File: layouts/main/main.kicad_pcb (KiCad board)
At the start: 4 copper layers, 20.5 x 20.5 mm, 60 parts

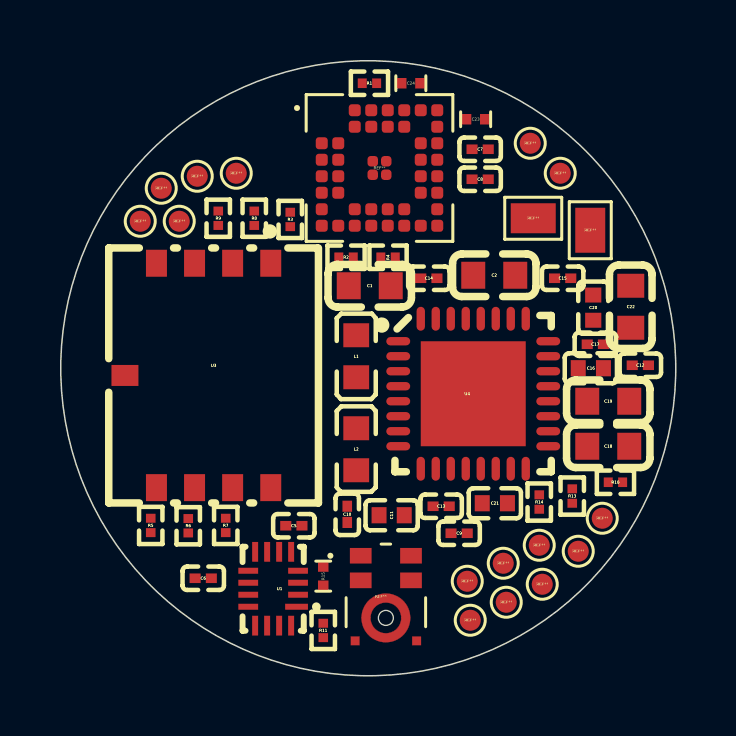
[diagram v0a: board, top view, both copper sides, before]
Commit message: wip
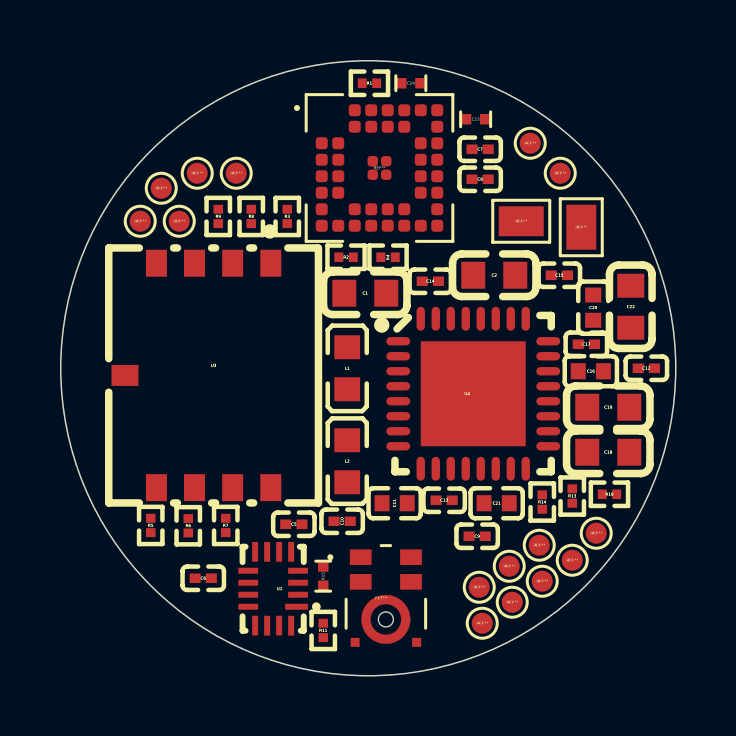
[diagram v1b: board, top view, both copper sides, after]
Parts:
- moved C9 0.61 mm to (3.63, 5.60)
- moved REF** 0.54 mm to (7.60, 5.50)
- moved L1 0.50 mm to (-0.70, 0.00)
- moved L2 0.50 mm to (-0.70, 3.10)
- moved R10 0.45 mm to (8.04, 4.20)
- moved REF** 0.45 mm to (3.70, 7.30)
- moved C11 0.41 mm to (0.88, 4.50)
- moved REF** 0.41 mm to (5.10, -4.90)
- moved REF** 0.41 mm to (3.80, 8.50)
- moved REF** 0.36 mm to (6.80, 6.40)
- moved REF** 0.32 mm to (7.10, -4.70)
- moved C17 0.30 mm to (7.27, -0.80)
- moved C1 0.29 mm to (-0.10, -2.50)
- moved C10 0.29 mm to (-0.87, 5.10), turned to 180 degrees
- moved REF** 0.22 mm to (4.70, 6.60)
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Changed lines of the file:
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@@
 	(footprint "POGO_PAD:POGO_PAD"
 		(layer "F.Cu")
-		(at 7.8 5)
+		(at 7.6 5.5)
 		(property "Reference" "REF**"
 			(at 0 0 0)
@@
 	(footprint "UNI_ROYAL_0201WMF0000TEE:R0201"
 		(layer "F.Cu")
-		(at 8.24 3.8)
+		(at 8.04 4.2)
 		(property "Reference" "R10"
 			(at 0 0 0)
@@
 	(footprint "UNI_ROYAL_0201WMF1002TEE:R0201"
 		(layer "F.Cu")
-		(at -3.8 -5 90)
+		(at -3.9 -5.06 90)
 		(property "Reference" "R8"
 			(at 0 0 0)
@@
 	(footprint "POGO_PAD:POGO_PAD"
 		(layer "F.Cu")
-		(at 3.3 7.1)
+		(at 3.7 7.3)
 		(property "Reference" "REF**"
 			(at 0 0 0)
@@
 	(footprint "Samsung_Electro_Mechanics_CL10A106KP8NNNC:C0603"
 		(layer "F.Cu")
-		(at 8 2.6)
+		(at 8 2.8)
 		(property "Reference" "C18"
 			(at 0 0 0)
@@
 	(footprint "Murata_Electronics_GRM033R60J104KE19D:C0201"
 		(layer "F.Cu")
-		(at -0.7 4.87 -90)
+		(at -0.87 5.1 180)
 		(property "Reference" "C10"
-			(at 0 -0.000167 0)
+			(at 0 -0.000167 90)
 			(layer "F.SilkS")
 			(effects
@@
 		)
 		(property "Value" "100nF ±10% X5R"
-			(at 0 -0.000167 0)
+			(at 0 -0.000167 90)
 			(layer "F.Fab")
 			(effects
@@
 		)
 		(property "Datasheet" "https://wmsc.lcsc.com/wmsc/upload/file/pdf/v2/lcsc/2304140030_Murata-Electronics-GRM033R60J104KE19D_C76928.pdf"
-			(at 0 0 90)
+			(at 0 0 0)
 			(layer "User.9")
 			(hide yes)
@@
 		)
 		(property "Description" ""
-			(at 0 0 90)
+			(at 0 0 0)
 			(layer "F.Fab")
 			(hide yes)
@@
 		)
 		(property "checksum" "4c698f746e469e1dee8eb9906937a259cc1e41bf0b356ab1e01eb74657f75796"
-			(at 0 0 0)
+			(at 0 0 90)
 			(layer "User.9")
 			(hide yes)
@@
 		)
 		(property "__atopile_lib_fp_hash__" "0fb5227f-9857-c04c-e64f-3cbb1c0819d1"
-			(at 0 0 0)
+			(at 0 0 90)
 			(layer "User.9")
 			(hide yes)
@@
 		)
 		(property "LCSC" "C76928"
-			(at 0 0 90)
+			(at 0 0 0)
 			(layer "User.9")
 			(hide yes)
@@
 		)
 		(property "Manufacturer" "Murata Electronics"
-			(at 0 0 90)
+			(at 0 0 0)
 			(layer "User.9")
 			(hide yes)
@@
 		)
 		(property "Partnumber" "GRM033R60J104KE19D"
-			(at 0 0 90)
+			(at 0 0 0)
 			(layer "User.9")
 			(hide yes)
@@
 		)
 		(property "PARAM_capacitance" "{\"type\": \"Quantity_Interval_Disjoint\", \"data\": {\"intervals\": {\"type\": \"Numeric_Interval_Disjoint\", \"data\": {\"intervals\": [{\"type\": \"Numeric_Interval\", \"data\": {\"min\": 9e-08, \"max\": 1.1e-07}}]}}, \"unit\": \"farad\"}}"
-			(at 0 0 90)
+			(at 0 0 0)
 			(layer "User.9")
 			(hide yes)
@@
 		)
 		(property "PARAM_max_voltage" "{\"type\": \"Quantity_Interval_Disjoint\", \"data\": {\"intervals\": {\"type\": \"Numeric_Interval_Disjoint\", \"data\": {\"intervals\": [{\"type\": \"Numeric_Interval\", \"data\": {\"min\": 0.0, \"max\": null}}]}}, \"unit\": \"volt\"}}"
-			(at 0 0 90)
+			(at 0 0 0)
 			(layer "User.9")
 			(hide yes)
@@
 		)
 		(property "PARAM_temperature_coefficient" "{\"type\": \"EnumSet\", \"data\": {\"elements\": [{\"name\": \"X5R\"}], \"enum\": {\"name\": \"TemperatureCoefficient\", \"values\": {\"Y5V\": 1, \"Z5U\": 2, \"X7S\": 3, \"X5R\": 4, \"X6R\": 5, \"X7R\": 6, \"X8R\": 7, \"C0G\": 8}}}}"
-			(at 0 0 90)
+			(at 0 0 0)
 			(layer "User.9")
 			(hide yes)
@@
 		)
 		(property "atopile_address" "c_nand"
-			(at 0 0 90)
+			(at 0 0 0)
 			(layer "User.9")
 			(hide yes)
@@
 		(attr through_hole)
 		(fp_line
-			(start -0.17 0.39)
-			(end -0.53 0.39)
+			(start 0.69 0.24)
+			(end 0.69 -0.24)
 			(stroke
 				(width 0.15)
@@
 		)
 		(fp_line
-			(start 0.17 0.39)
-			(end 0.53 0.39)
+			(start 0.53 -0.39)
+			(end 0.17 -0.39)
 			(stroke
 				(width 0.15)
@@
 		)
 		(fp_line
-			(start -0.69 0.24)
-			(end -0.69 -0.24)
+			(start 0.17 0.39)
+			(end 0.53 0.39)
 			(stroke
 				(width 0.15)
@@
 		)
 		(fp_line
-			(start 0.69 0.24)
-			(end 0.69 -0.24)
+			(start -0.17 0.39)
+			(end -0.53 0.39)
 			(stroke
 				(width 0.15)
@@
 		)
 		(fp_line
-			(start 0.53 -0.39)
-			(end 0.17 -0.39)
+			(start -0.69 0.24)
+			(end -0.69 -0.24)
 			(stroke
 				(width 0.15)
@@
 		)
 		(fp_arc
-			(start -0.529667 0.389644)
-			(mid -0.642347 0.349658)
-			(end -0.69 0.24)
+			(start 0.69 0.24)
+			(mid 0.642348 0.349658)
+			(end 0.529667 0.389644)
 			(stroke
 				(width 0.15)
@@
 		)
 		(fp_arc
-			(start 0.69 0.24)
-			(mid 0.642348 0.349658)
-			(end 0.529667 0.389644)
+			(start 0.53 -0.39)
+			(mid 0.642835 -0.349658)
+			(end 0.690333 -0.239643)
 			(stroke
 				(width 0.15)
@@
 		)
 		(fp_arc
-			(start -0.690333 -0.239643)
-			(mid -0.642835 -0.349658)
-			(end -0.53 -0.39)
+			(start -0.529667 0.389644)
+			(mid -0.642347 0.349658)
+			(end -0.69 0.24)
 			(stroke
 				(width 0.15)
@@
 		)
 		(fp_arc
-			(start 0.53 -0.39)
-			(mid 0.642835 -0.349658)
-			(end 0.690333 -0.239643)
+			(start -0.690333 -0.239643)
+			(mid -0.642835 -0.349658)
+			(end -0.53 -0.39)
 			(stroke
 				(width 0.15)
@@
 		)
 		(fp_text user "${REFERENCE}"
-			(at 0 -0.000167 0)
+			(at 0 -0.000167 90)
 			(layer "F.SilkS")
 			(effects
@@
 		)
 		(fp_text user "${REFERENCE}"
-			(at 0 -0.000167 0)
+			(at 0 -0.000167 90)
 			(layer "F.Fab")
 			(effects
@@
 		)
 		(pad "1" smd rect
-			(at -0.27 0 270)
+			(at -0.27 0 180)
 			(size 0.37 0.32)
 			(layers "F.Cu" "F.Mask" "F.Paste")
@@
 		)
 		(pad "2" smd rect
-			(at 0.27 0 270)
+			(at 0.27 0 180)
 			(size 0.37 0.32)
 			(layers "F.Cu" "F.Mask" "F.Paste")
@@
 	(footprint "Murata_Electronics_GRM033R60J104KE19D:C0201"
 		(layer "F.Cu")
-		(at 3.03 5.5)
+		(at 3.63 5.6)
 		(property "Reference" "C9"
 			(at 0 -0.000167 0)
@@
 	(footprint "POGO_PAD:POGO_PAD"
 		(layer "F.Cu")
-		(at 7 6.1)
+		(at 6.8 6.4)
 		(property "Reference" "REF**"
 			(at 0 0 0)
@@
 	(footprint "YAGEO_RC0201FR_07150KL:R0201"
 		(layer "F.Cu")
-		(at 5.7 4.46 -90)
+		(at 5.8 4.46 -90)
 		(property "Reference" "R14"
 			(at 0 0 0)
@@
 	(footprint "Murata_Electronics_GRM033R60J104KE19D:C0201"
 		(layer "F.Cu")
-		(at 2.02 -3)
+		(at 2.07 -2.9)
 		(property "Reference" "C14"
 			(at 0 -0.000167 0)
@@
 	(footprint "FH_CMH160808B2R2MT:L0603"
 		(layer "F.Cu")
-		(at -0.4 -0.4 90)
+		(at -0.7 0 90)
 		(property "Reference" "L1"
 			(at -0.005 0 0)
@@
 	(footprint "Murata_Electronics_GRM033R60J104KE19D:C0201"
 		(layer "F.Cu")
-		(at 2.43 4.6 180)
+		(at 2.53 4.4 180)
 		(property "Reference" "C13"
 			(at 0 -0.000166 0)
@@
 	(footprint "POGO_PAD:POGO_PAD"
 		(layer "F.Cu")
-		(at 4.6 7.8)
+		(at 4.8 7.8)
 		(property "Reference" "REF**"
 			(at 0 0 0)
@@
 	(footprint "UNI_ROYAL_0201WMF4701TEE:R0201"
 		(layer "F.Cu")
-		(at -2.6 -4.96 -90)
+		(at -2.7 -5.06 -90)
 		(property "Reference" "R3"
 			(at 0 0 0)
@@
 	(footprint "POGO_PAD:POGO_PAD"
 		(layer "F.Cu")
-		(at -5.7 -6.4)
+		(at -5.7 -6.5)
 		(property "Reference" "REF**"
 			(at 0 0 0)
@@
 	(footprint "Samsung_Electro_Mechanics_CL05A225MQ5NSNC:C0402"
 		(layer "F.Cu")
-		(at 0.78 4.9)
+		(at 0.88 4.5)
 		(property "Reference" "C11"
 			(at 0 0 90)
@@
 	(footprint "POGO_PAD:POGO_PAD"
 		(layer "F.Cu")
-		(at 4.5 6.5)
+		(at 4.7 6.6)
 		(property "Reference" "REF**"
 			(at 0 0 0)
@@
 	(footprint "Samsung_Electro_Mechanics_CL05A105KA5NQNC:C0402"
 		(layer "F.Cu")
-		(at 4.22 4.5)
+		(at 4.28 4.5)
 		(property "Reference" "C21"
 			(at 0 0 0)
@@
 	(footprint "FH_CMH160808B2R2MT:L0603"
 		(layer "F.Cu")
-		(at -0.4 2.7 -90)
+		(at -0.7 3.1 -90)
 		(property "Reference" "L2"
 			(at -0.005 0 0)
@@
 	(footprint "INVENSENSE_MMICT5838_00_012:MIC_T5838"
 		(layer "F.Cu")
-		(at 0.5875 7.612)
+		(at 0.5875 7.662)
 		(property "Reference" "REF**"
 			(at -0.1625 0 0)
@@
 	(footprint "Samsung_Electro_Mechanics_CL05A105KA5NQNC:C0402"
 		(layer "F.Cu")
-		(at 7.42 0)
+		(at 7.42 0.1)
 		(property "Reference" "C16"
 			(at 0 0 0)
@@
 	(footprint "Murata_Electronics_GRM033R60J104KE19D:C0201"
 		(layer "F.Cu")
-		(at 9.07 -0.1)
+		(at 9.27 0)
 		(property "Reference" "C12"
 			(at 0 -0.000167 0)
@@
 	(footprint "Samsung_Electro_Mechanics_CL10A106KP8NNNC:C0603"
 		(layer "F.Cu")
-		(at 8 1.1)
+		(at 8 1.3)
 		(property "Reference" "C19"
 			(at 0 0 0)
@@
 	(footprint "BATTERY_PAD:BATTERY_PAD"
 		(layer "F.Cu")
-		(at 7.4 -4.6 180)
+		(at 7.1 -4.7 180)
 		(property "Reference" "REF**"
 			(at 0 0 0)
@@
 	(footprint "POGO_PAD:POGO_PAD"
 		(layer "F.Cu")
-		(at 3.4 8.4)
+		(at 3.8 8.5)
 		(property "Reference" "REF**"
 			(at 0 0 0)
@@
 	(footprint "Murata_Electronics_GRM033R60J104KE19D:C0201"
 		(layer "F.Cu")
-		(at 6.48 -3)
+		(at 6.37 -3.1)
 		(property "Reference" "C15"
 			(at 0 -0.000167 0)
@@
 	(footprint "POGO_PAD:POGO_PAD"
 		(layer "F.Cu")
-		(at 5.8 7.2)
+		(at 5.8 7.1)
 		(property "Reference" "REF**"
 			(at 0 0 0)
@@
 	(footprint "Samsung_Electro_Mechanics_CL10A106KP8NNNC:C0603"
 		(layer "F.Cu")
-		(at 0.05 -2.75)
+		(at -0.1 -2.5)
 		(property "Reference" "C1"
 			(at 0 0 0)
@@
 	(footprint "Murata_Electronics_GRM033R60J104KE19D:C0201"
 		(layer "F.Cu")
-		(at 7.57 -0.8)
+		(at 7.27 -0.8)
 		(property "Reference" "C17"
 			(at 0 -0.000167 0)
@@
 	(footprint "Murata_Electronics_GRM033R60J104KE19D:C0201"
 		(layer "F.Cu")
-		(at -2.48 5.25)
+		(at -2.48 5.2)
 		(property "Reference" "C5"
 			(at 0 -0.000167 0)
@@
 	(footprint "UNI_ROYAL_0201WMF1002TEE:R0201"
 		(layer "F.Cu")
-		(at -5 -5 90)
+		(at -5 -5.06 90)
 		(property "Reference" "R9"
 			(at 0 0 0)
@@
 	(footprint "BATTERY_PAD:BATTERY_PAD"
 		(layer "F.Cu")
-		(at 5.5 -5 -90)
+		(at 5.1 -4.9 -90)
 		(property "Reference" "REF**"
 			(at 0 0 0)

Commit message: drc rules
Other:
- rule pad_to_mask_clearance: 0 -> 0.05
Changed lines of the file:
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@@
 			(dielectric_constraints no)
 		)
-		(pad_to_mask_clearance 0)
+		(pad_to_mask_clearance 0.05)
+		(solder_mask_min_width 0.1)
 		(allow_soldermask_bridges_in_footprints no)
 		(tenting front back)

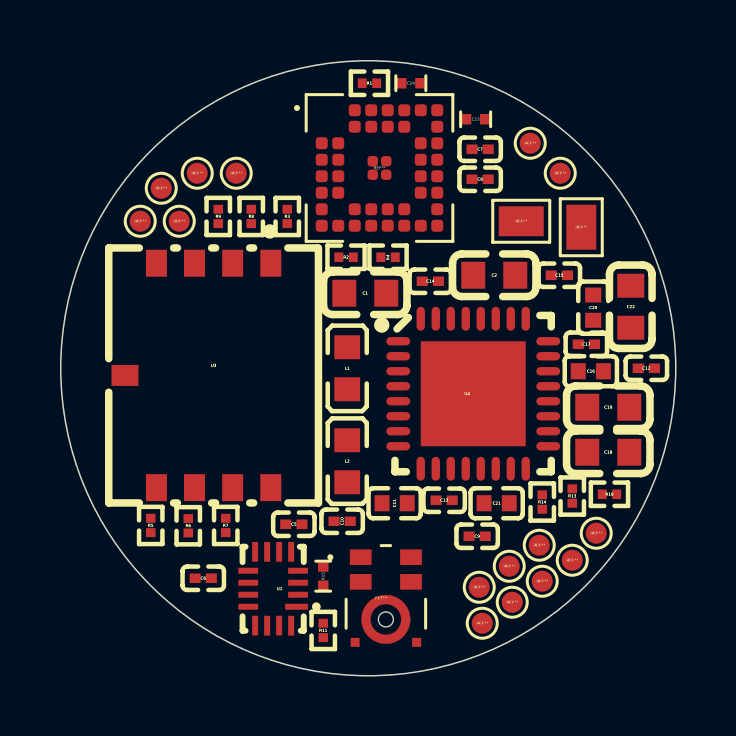
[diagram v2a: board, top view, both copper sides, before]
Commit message: wip
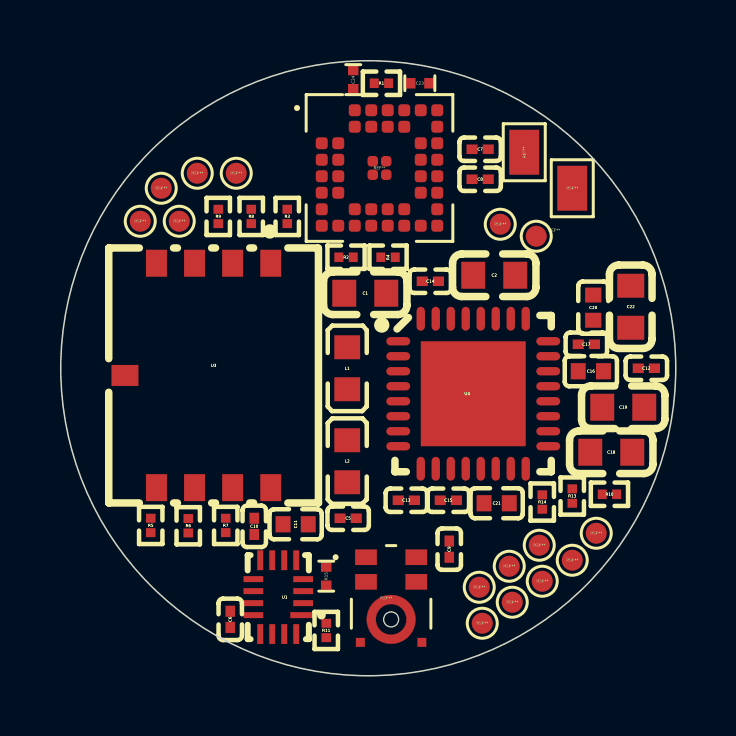
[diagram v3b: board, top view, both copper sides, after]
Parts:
- moved C15 8.36 mm to (2.67, 4.40), turned to 180 degrees
- moved C11 3.37 mm to (-2.42, 5.20)
- moved REF** 3.11 mm to (5.60, -4.40)
- moved C10 2.93 mm to (-3.80, 5.27), turned to 90 degrees
- moved REF** 2.62 mm to (4.40, -4.80)
- moved REF** 2.30 mm to (5.20, -7.20), turned to 0 degrees
- moved C23 2.21 mm to (1.72, -9.50)
- moved C24 1.92 mm to (-0.50, -9.62), turned to 90 degrees
- moved C5 1.82 mm to (-0.67, 5.00)
- moved C6 1.64 mm to (-4.60, 8.37), turned to 90 degrees
- moved REF** 1.33 mm to (6.80, -6.00)
- moved C13 1.26 mm to (1.27, 4.40)
- moved C9 1.02 mm to (2.70, 6.03), turned to 90 degrees
- moved C19 0.50 mm to (8.50, 1.30)
- moved R1 0.40 mm to (0.44, -9.50)
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
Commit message: wip
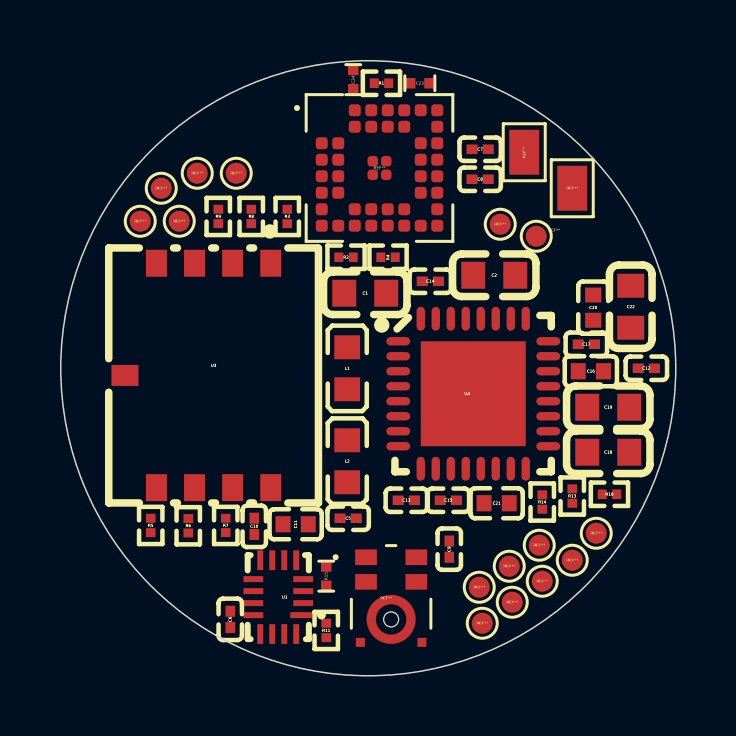
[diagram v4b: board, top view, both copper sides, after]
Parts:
- moved C19 0.50 mm to (8.00, 1.30)
- moved C18 0.10 mm to (8.00, 2.80)
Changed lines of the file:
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@@
 	(footprint "Samsung_Electro_Mechanics_CL10A106KP8NNNC:C0603"
 		(layer "F.Cu")
-		(at 8.1 2.8)
+		(at 8 2.8)
 		(property "Reference" "C18"
 			(at 0 0 0)
@@
 	(footprint "Samsung_Electro_Mechanics_CL10A106KP8NNNC:C0603"
 		(layer "F.Cu")
-		(at 8.5 1.3)
+		(at 8 1.3)
 		(property "Reference" "C19"
 			(at 0 0 0)
